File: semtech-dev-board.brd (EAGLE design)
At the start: 58.1 x 96.4 mm, 58 parts, among them Q1 BSS123, U1 SEMTECH_SX1236, U3 MIC5219 3.3V, X1 BU-SMA-G, X2 BU-SMA-G, X3 BU-SMA-G, X4 BU-SMA-G

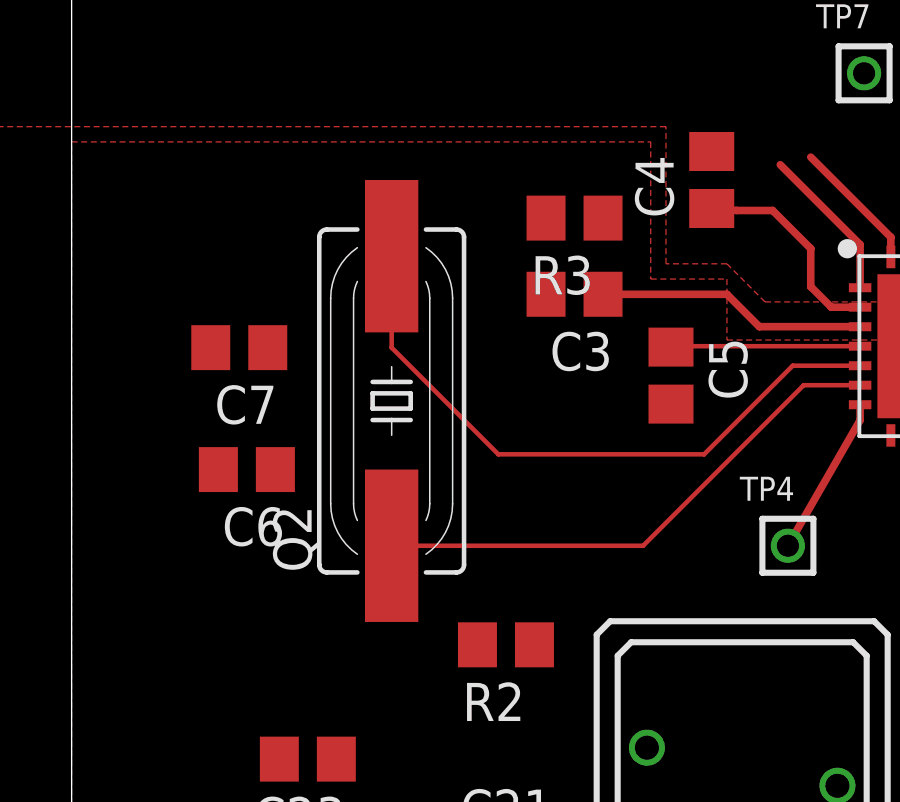
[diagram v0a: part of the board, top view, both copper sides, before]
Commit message: minor edits
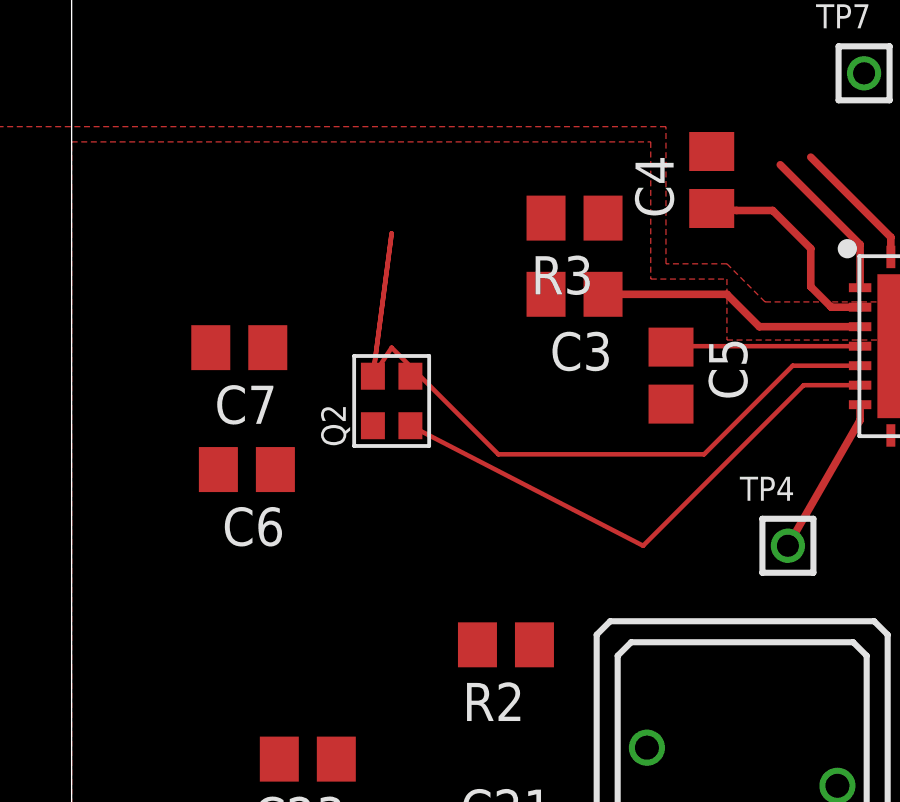
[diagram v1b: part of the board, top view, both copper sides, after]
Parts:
- Q2: device crystal:SM49 -> low-gain-radio:CRYSTAL_2.5X2
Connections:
- net N$2: now also Q2.3; no longer Q2.2
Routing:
- net N$2: track 22.9 -> 29.1 mm
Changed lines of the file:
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@@
 <element name="LED1" library="led" package="CHIP-LED0805" value="" x="38.1" y="5.588" rot="R270"/>
 <element name="Q1" library="transistor-small-signal" package="SOT23" value="BSS123" x="42.672" y="10.668" rot="R90"/>
-<element name="Q2" library="crystal" package="SM49" value="" x="27.686" y="32.258" rot="R90">
-<attribute name="MF" value="" x="27.686" y="32.258" size="1.778" layer="27" rot="R90" display="off"/>
-<attribute name="MPN" value="" x="27.686" y="32.258" size="1.778" layer="27" rot="R90" display="off"/>
-<attribute name="OC_FARNELL" value="unknown" x="27.686" y="32.258" size="1.778" layer="27" rot="R90" display="off"/>
-<attribute name="OC_NEWARK" value="unknown" x="27.686" y="32.258" size="1.778" layer="27" rot="R90" display="off"/>
-</element>
+<element name="Q2" library="low-gain-radio" package="CRYSTAL_2.5X2" value="" x="27.686" y="32.258" rot="R90"/>
 <element name="R1" library="rcl" package="M0805" value="" x="37.592" y="10.668" rot="R90"/>
 <element name="R2" library="rcl" package="R0805" value="1k" x="31.496" y="24.13" rot="R180"/>
@@
 <wire x1="43.301" y1="32.784" x2="41.42" y2="32.784" width="0.1524" layer="1"/>
 <wire x1="41.42" y1="32.784" x2="36.068" y2="27.432" width="0.1524" layer="1"/>
-<wire x1="36.068" y1="27.432" x2="27.686" y2="27.432" width="0.1524" layer="1"/>
-<wire x1="27.686" y1="27.432" x2="23.81" y2="29.972" width="0" layer="19" extent="1-1"/>
+<wire x1="36.068" y1="27.432" x2="28.311" y2="31.433" width="0.1524" layer="1"/>
+<wire x1="28.311" y1="31.433" x2="23.81" y2="29.972" width="0" layer="19" extent="1-1"/>
 </signal>
 <signal name="RXTX">
@@
 <signal name="N$2">
 <contactref element="U1" pad="5"/>
-<contactref element="Q2" pad="2"/>
+<contactref element="Q2" pad="3"/>
 <contactref element="C7" pad="1"/>
 <wire x1="43.301" y1="33.434" x2="41.054" y2="33.434" width="0.1524" layer="1"/>
@@
 <wire x1="38.1" y1="30.48" x2="31.242" y2="30.48" width="0.1524" layer="1"/>
 <wire x1="31.242" y1="30.48" x2="27.686" y2="34.036" width="0.1524" layer="1"/>
-<wire x1="27.686" y1="34.036" x2="27.686" y2="37.084" width="0.1524" layer="1"/>
-<wire x1="27.686" y1="37.846" x2="27.686" y2="37.084" width="0.1524" layer="1"/>
-<wire x1="27.686" y1="37.084" x2="27.686" y2="37.846" width="0.1524" layer="1"/>
+<wire x1="27.686" y1="34.036" x2="27.061" y2="33.083" width="0.1524" layer="1"/>
+<wire x1="27.686" y1="37.846" x2="27.061" y2="33.083" width="0.1524" layer="1"/>
+<wire x1="27.061" y1="33.083" x2="27.686" y2="37.846" width="0.1524" layer="1"/>
 <wire x1="23.556" y1="34.036" x2="27.686" y2="34.036" width="0" layer="19" extent="1-1"/>
 </signal>
